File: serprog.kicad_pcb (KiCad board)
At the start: 2 copper layers, 53 x 23.5 mm, 44 parts, among them J1 USB_B_Micro, J2 Conn_01x04, SW1 SW_Push_SPDT, U1 TXS0108EPW, U2 XC6206PxxxMR1v8, U3 XC6206PxxxMR3v3, U4 AT25xxx, U5 STM32F102R8Tx, Y1 8M

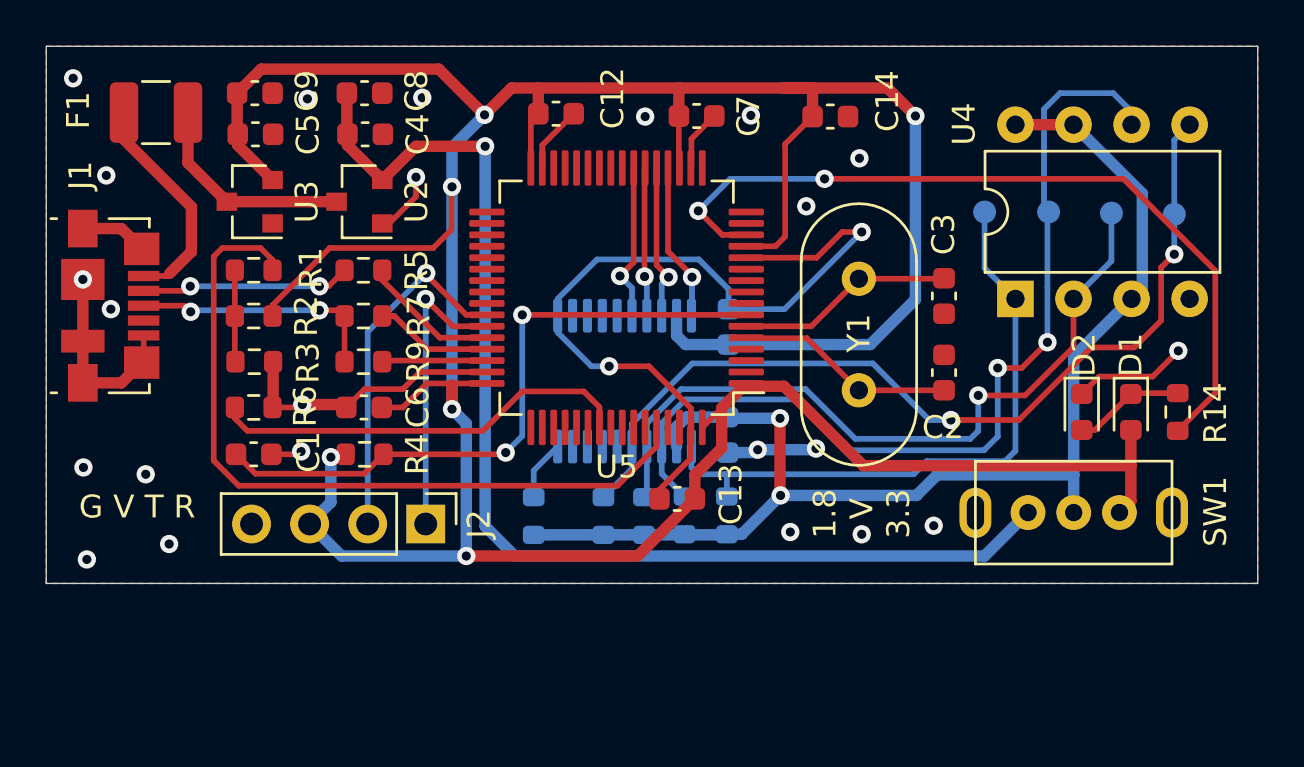
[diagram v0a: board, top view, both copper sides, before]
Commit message: v0.1
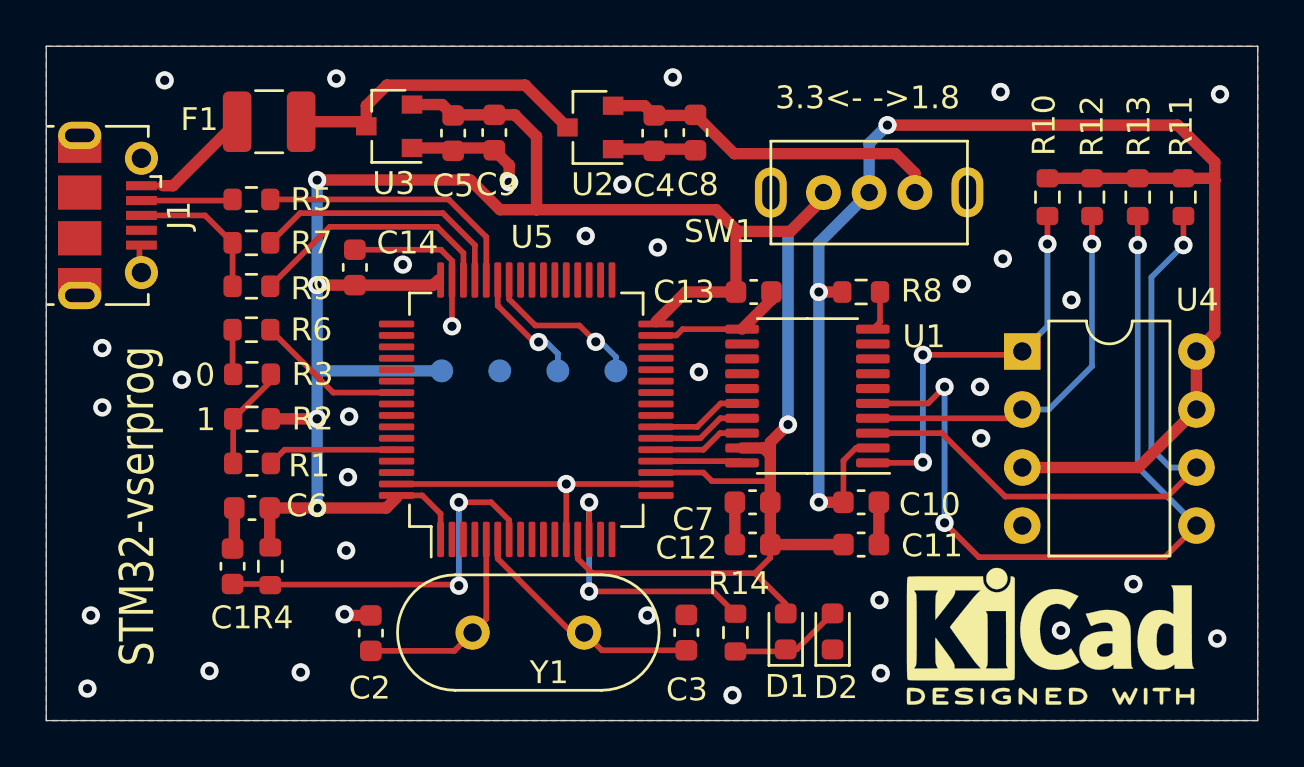
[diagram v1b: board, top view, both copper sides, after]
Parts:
- removed J2: Conn_01x04, Connector_PinHeader_2.54mm:PinHeader_1x04_P2.54mm_Vertical
- removed TP1, TP2, TP3, TP4: TestPoint, TestPoint:TestPoint_Pad_D1.0mm
- added 3V3: TestPoint, TestPoint:TestPoint_Pad_D1.0mm, B.Cu at (119.4, 70.0)
- added G: TestPoint, TestPoint:TestPoint_Pad_D1.0mm, B.Cu at (121.9, 70.0)
- added REF**: KiCad-Logo2_5mm_SilkScreen, Symbol:KiCad-Logo2_5mm_SilkScreen, F.Cu at (146.0, 81.6)
- added RX: TestPoint, TestPoint:TestPoint_Pad_D1.0mm, B.Cu at (124.5, 70.0)
- added TX: TestPoint, TestPoint:TestPoint_Pad_D1.0mm, B.Cu at (127.0, 70.0)
- C10, C11, R10, R11, R12, R13, R8, U1: moved to F.Cu
- J1: footprint Connector_USB:USB_Micro-B_Molex_47346-0001 -> Connector_USB:USB_Micro-B_Molex-105017-0001
- moved C2 27.5 mm to (116.3, 81.5)
- moved R13 27.2 mm to (149.8, 62.4), turned to 270 degrees
- moved R11 25.9 mm to (151.8, 62.4), turned to 270 degrees
- moved R12 24.1 mm to (147.8, 62.4), turned to 270 degrees
- moved C14 21.8 mm to (115.6, 65.5), turned to 90 degrees
- moved R14 21.6 mm to (132.2, 81.5), turned to 270 degrees
- moved C12 20.7 mm to (133.0, 77.6), turned to 180 degrees
- moved SW1 20.0 mm to (133.8, 64.5), turned to 90 degrees
- moved Y1 19.9 mm to (120.8, 81.5), turned to 0 degrees
- moved R10 19.8 mm to (145.9, 62.4), turned to 270 degrees
- moved C3 18.5 mm to (130.1, 81.5), turned to 90 degrees
- moved D1 17.9 mm to (134.4, 81.4), turned to 90 degrees
- moved R8 17.4 mm to (137.8, 66.5), turned to 0 degrees
- moved C7 17.1 mm to (133.0, 75.8), turned to 180 degrees
- moved C8 14.6 mm to (130.5, 59.6), turned to 270 degrees
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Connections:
- SW1 pad : GND -> (no net)
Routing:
- net +3V3: track 165.0 -> 116.8 mm, vias 6 -> 5
- net +1V8: track 51.3 -> 15.3 mm, vias 1 -> 0
- net GND: track 78.1 -> 45.9 mm, vias 25 -> 36
- net BOOT0: track 33.7 -> 5.75 mm
- net PA0: track 35.1 -> 12.3 mm
- net FLASH_MISO: track 32.6 -> 17.1 mm
- net FLASH_SCK: track 41.4 -> 28.9 mm, vias 2 -> 1
- net BOOT1: track 18.5 -> 6.66 mm
- net nRST: track 28.7 -> 17.0 mm
- net FLASH_NSS: track 27.7 -> 17.7 mm, vias 0 -> 3
- net FLASH_VCC: track 55.7 -> 65.4 mm, vias 2 -> 3
- net USART1_TX: track 15.5 -> 7.17 mm
- net USART1_RX: track 13.0 -> 5.37 mm
- net PA13: track 4.60 -> 11.2 mm
- net USBDP: track 5.18 -> 11.6 mm
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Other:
- board size 53 x 23.5 mm -> 53 x 29.5 mm
- board text added: "0"
- board text added: "1"
- board text added: "3.3<- ->1.8"
- board text added: "STM32-vserprog"
- board text removed: "1.8 V 3.3"
- board text removed: "G V T R"
